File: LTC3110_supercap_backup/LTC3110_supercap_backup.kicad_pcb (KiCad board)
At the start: 2 copper layers, 30 parts, among them M1 2N7002, M2 2N7002, P1 CONN_01X02, P2 CONN_01X02, P3 CONN_01X05, Q1 Q_PNP_BCEC, U1 LTC2935-2-TS8, U2 LTC3110EFE

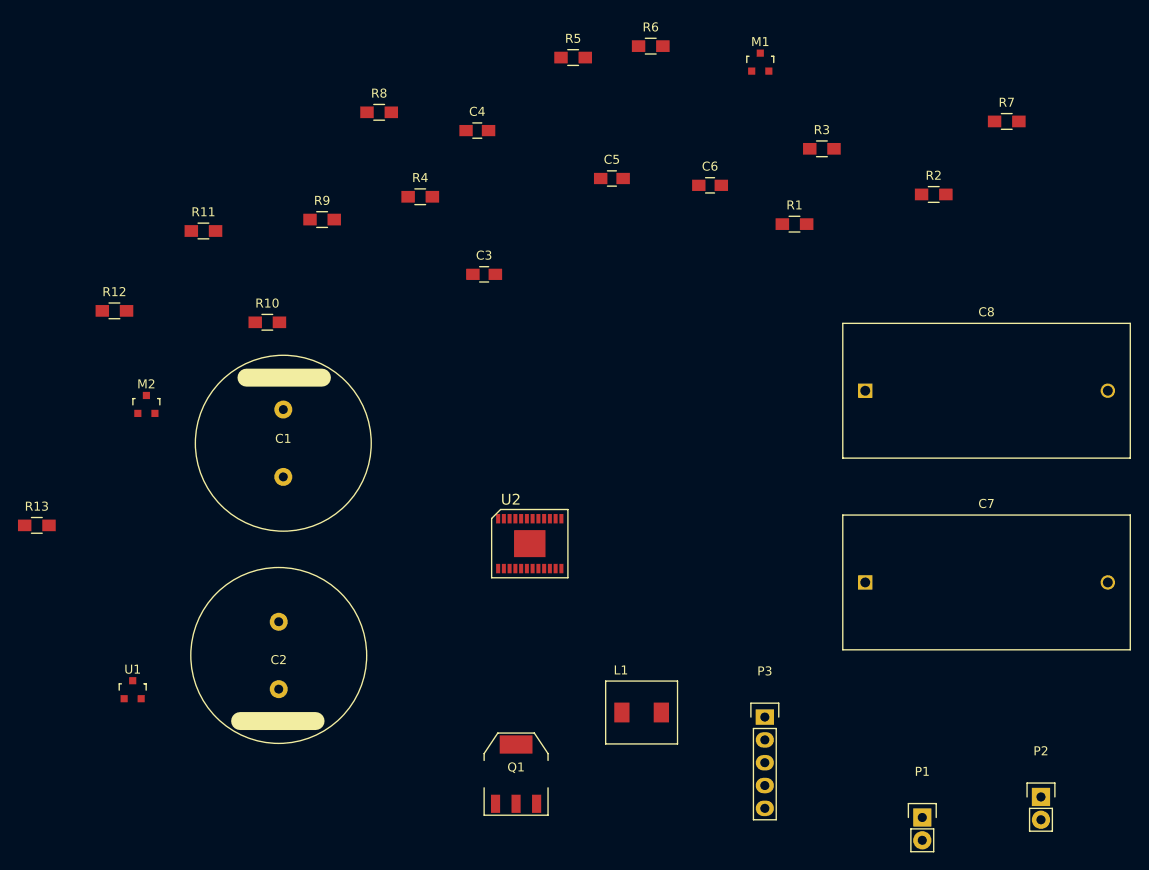
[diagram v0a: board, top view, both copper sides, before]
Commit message: Layout almost complete
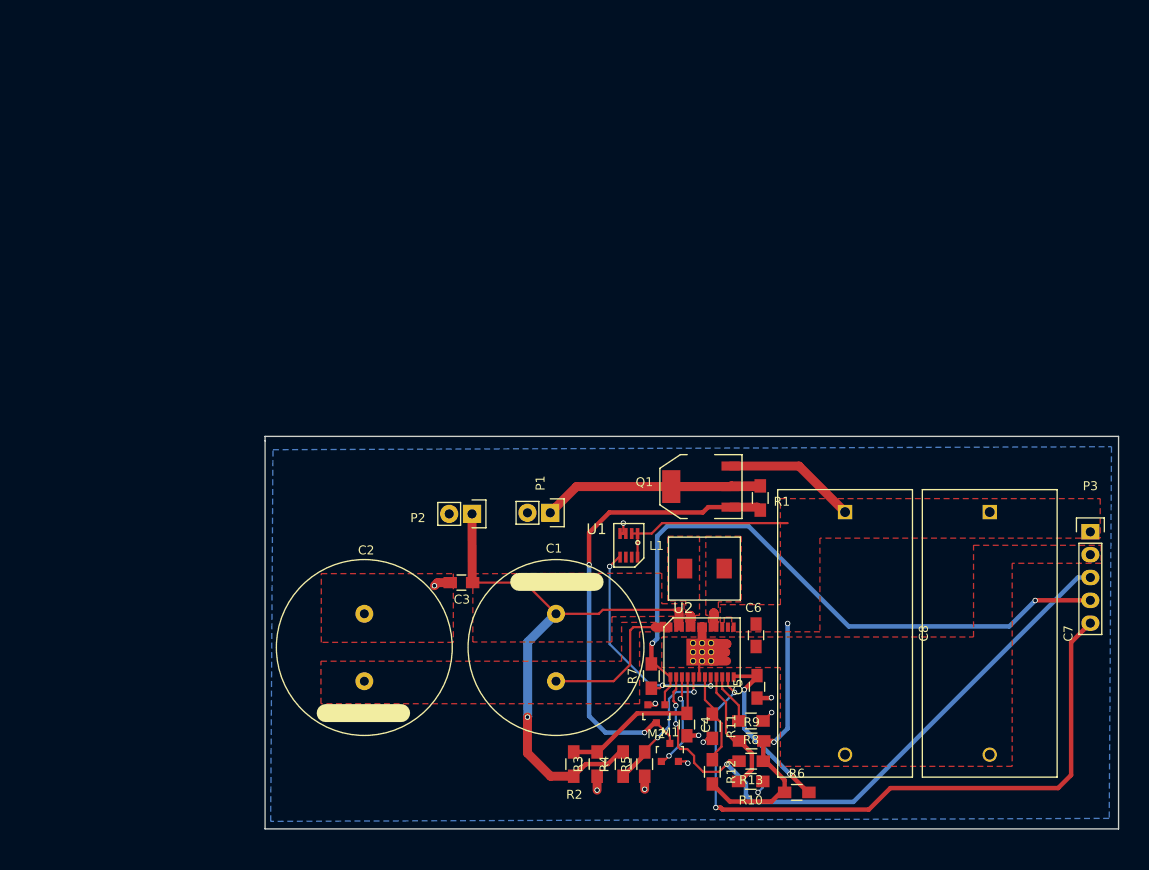
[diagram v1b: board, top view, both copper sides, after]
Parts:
- U1: footprint TO_SOT_Packages_SMD:SOT-23 -> MRV_SMD_Packages:TSOT-23-8
- moved R6 84.6 mm to (157.2, 142.7)
- moved R12 84.0 mm to (147.8, 140.5), turned to 270 degrees
- moved R13 83.7 mm to (152.2, 139.3), turned to 180 degrees
- moved R8 79.4 mm to (152.1, 134.8), turned to 180 degrees
- moved R5 79.0 mm to (140.3, 139.6), turned to 90 degrees
- moved R11 79.0 mm to (147.8, 135.4), turned to 270 degrees
- moved M1 77.5 mm to (143.1, 138.3)
- moved R9 75.2 mm to (152.2, 137.0)
- moved R2 75.0 mm to (132.4, 139.6), turned to 90 degrees
- moved R10 74.2 mm to (152.1, 141.5), turned to 180 degrees
- moved R7 73.3 mm to (141.0, 129.8), turned to 90 degrees
- moved R3 72.9 mm to (135.0, 139.6), turned to 90 degrees
- moved P2 70.7 mm to (121.1, 111.8), turned to 270 degrees
- moved C4 70.1 mm to (145.0, 135.2), turned to 270 degrees
- moved R4 67.1 mm to (137.9, 139.6), turned to 90 degrees
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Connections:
- C3 pad 1: Net-(C3-Pad1) -> /VCAP
- R12 pad 2: Net-(R12-Pad2) -> V_SYS
- R13 pad 1: Net-(R12-Pad2) -> V_SYS
- R9 pad 2: Net-(R12-Pad2) -> V_SYS
- U2 pad 25: (no net) -> GND
- U2 pad 6: GNDA -> GND
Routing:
- net CAP_OK: track 0.00 -> 75.0 mm, vias 0 -> 2
- net !CHRG: track 0.00 -> 74.8 mm, vias 0 -> 2
- net CAP_LOW: track 0.00 -> 71.9 mm, vias 0 -> 3
- net V_SYS: track 0.00 -> 66.5 mm, vias 0 -> 2
- net /VCAP: track 0.00 -> 65.5 mm, vias 0 -> 1
- net Net-(M1-Pad3): track 0.00 -> 52.4 mm, vias 0 -> 2
- net V_SOLAR: track 0.00 -> 34.6 mm
- net GND: track 0.00 -> 33.9 mm, vias 0 -> 10
- net /RUN: track 0.00 -> 25.8 mm, vias 0 -> 3
- net Net-(C5-Pad2): track 0.00 -> 21.9 mm, vias 0 -> 2
- net Net-(C4-Pad1): track 0.00 -> 18.9 mm
- net /V_MID: track 0.00 -> 18.7 mm
- net /FBVCAP: track 0.00 -> 15.5 mm, vias 0 -> 2
- net /FB: track 0.00 -> 14.3 mm
- net /MODE: track 0.00 -> 10.9 mm, vias 0 -> 2
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- added copper zone on F.Cu, net /VCAP
- added copper zone on F.Cu, net /V_MID
- added copper zone on B.Cu, net GND
- added copper zone on F.Cu, net GND
- added copper zone on F.Cu, net Net-(L1-Pad1)
- added copper zone on F.Cu, net Net-(L1-Pad2)
- added copper zone on F.Cu, net V_SYS
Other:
- board outline added: 95 x 43.7 mm
